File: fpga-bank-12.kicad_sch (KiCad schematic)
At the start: 1 part, among them U4 XC7K160T-FFG676

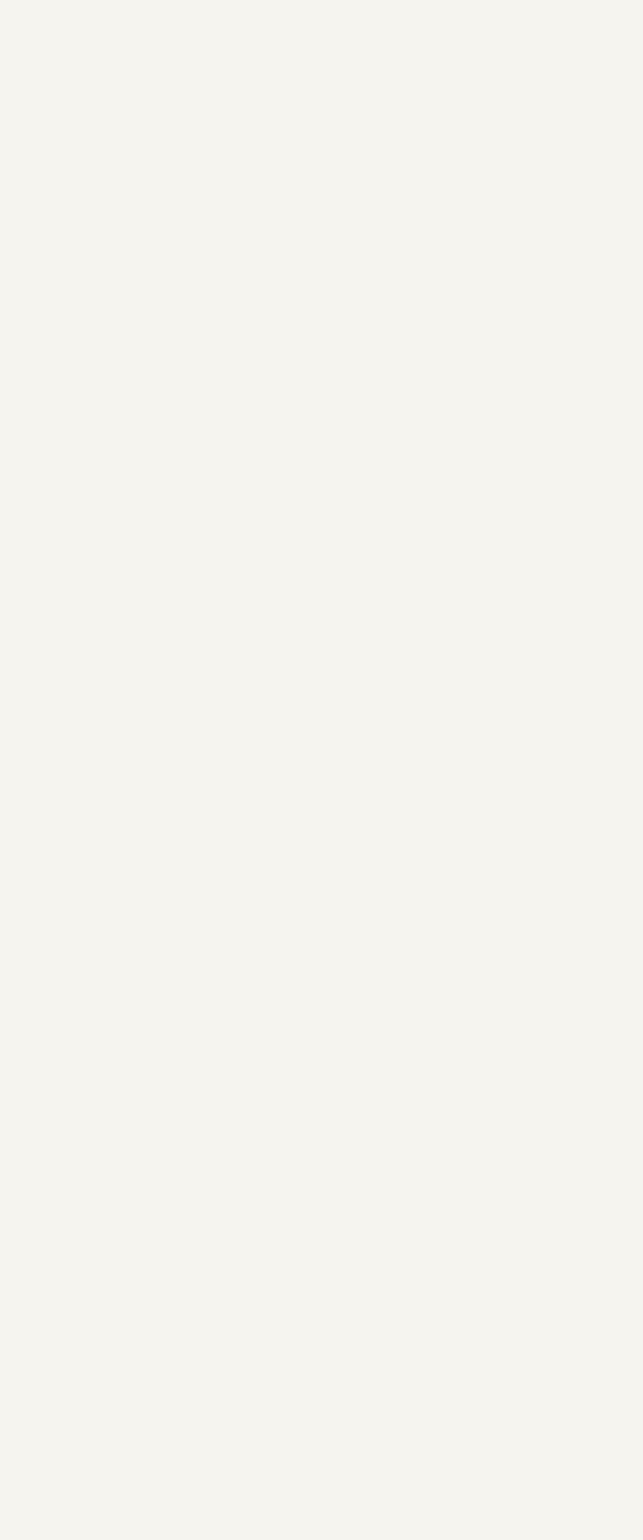
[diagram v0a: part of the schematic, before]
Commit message: [#65754] Rename project
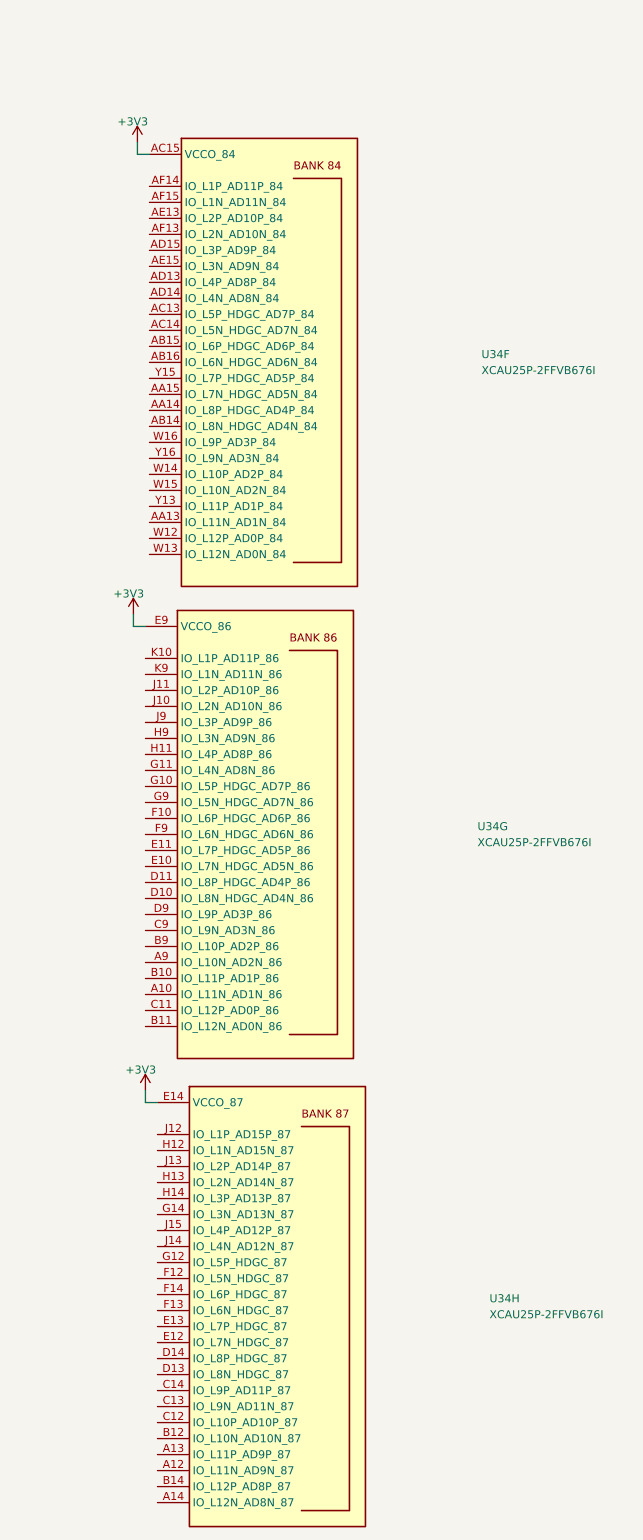
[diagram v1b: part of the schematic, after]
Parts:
- added U34: XCAU25P-2FFVB676I, antmicro-footprints:BGA-676_27x27mm_Layout26x26_P1x1mm_FFVB676, symbol antmicroFPGAChips:XCAU25P-2FFVB676I
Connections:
- net +3V3: now also U34.AC15 (VCCO_84), U34.E14 (VCCO_87), U34.E9 (VCCO_86), U34.H10 (VCCO_86), U34.H15 (VCCO_87), U34.Y14 (VCCO_84)
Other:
- title: SO-DIMM DDR5 Tester -> RDIMM DDR5 Tester
